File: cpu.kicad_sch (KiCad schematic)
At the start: 36 parts, among them J11 Debug, J12 GPS_Snoop, J13 I2C_Snoop, J6 USB_C_Receptacle_16P, U4 STM32H503KBUx, Y1 32768Hz

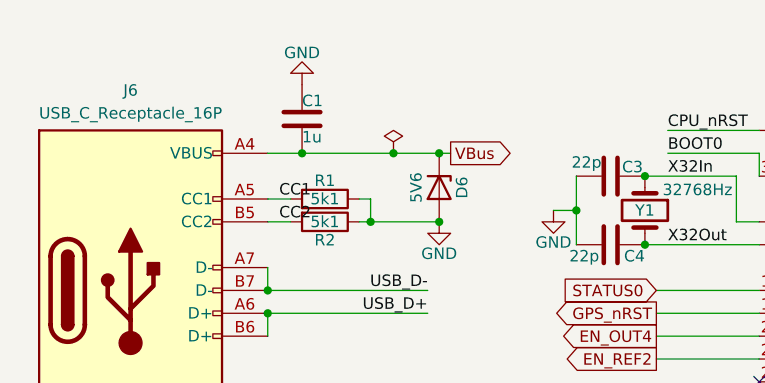
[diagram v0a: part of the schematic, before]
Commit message: Down to the dregs and clean-ups.
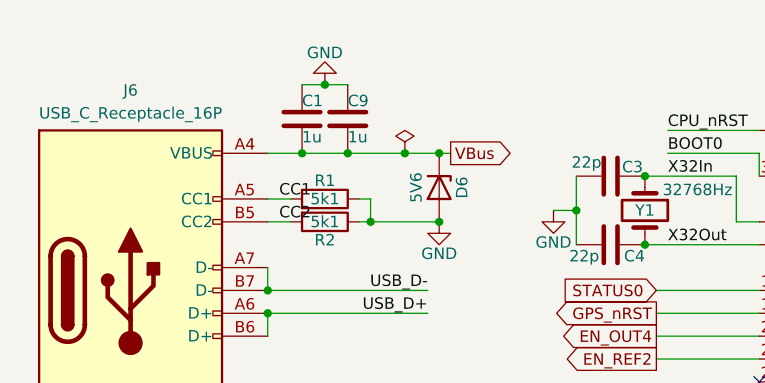
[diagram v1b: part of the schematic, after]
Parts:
- added C9: 1u, Capacitor_SMD:C_0402_1005Metric, symbol Device:C
- C1: JLCPCB (none) -> C52923
- C5: JLCPCB (none) -> C15195
- C6, C7, C8: JLCPCB (none) -> C307331
- D1, D2, D5, J13: now left out of the parts list
- R1, R2: JLCPCB (none) -> C25905
- R17, R18, R25: JLCPCB (none) -> C25744
- R20, R21, R3, R4, R5, R6, R7, R8, R9: JLCPCB (none) -> C25076
- R22, R23, R24: JLCPCB (none) -> C11702
- U4: JLCPCB (none) -> C22385521
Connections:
- net GND: now also C9.1
- net VBus: now also C9.2
